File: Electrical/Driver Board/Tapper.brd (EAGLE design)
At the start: 71.9 x 31.4 mm, 30 parts, among them CN1 1X4-BIG, U10 DRV2605LDGS, U11 DRV2605LDGS, U12 TCA9548APWR, U3 DRV2605LDGS, U4 DRV2605LDGS, U5 DRV2605LDGS, U6 DRV2605LDGS, U7 DRV2605LDGS, U8 DRV2605LDGS, U9 DRV2605LDGS

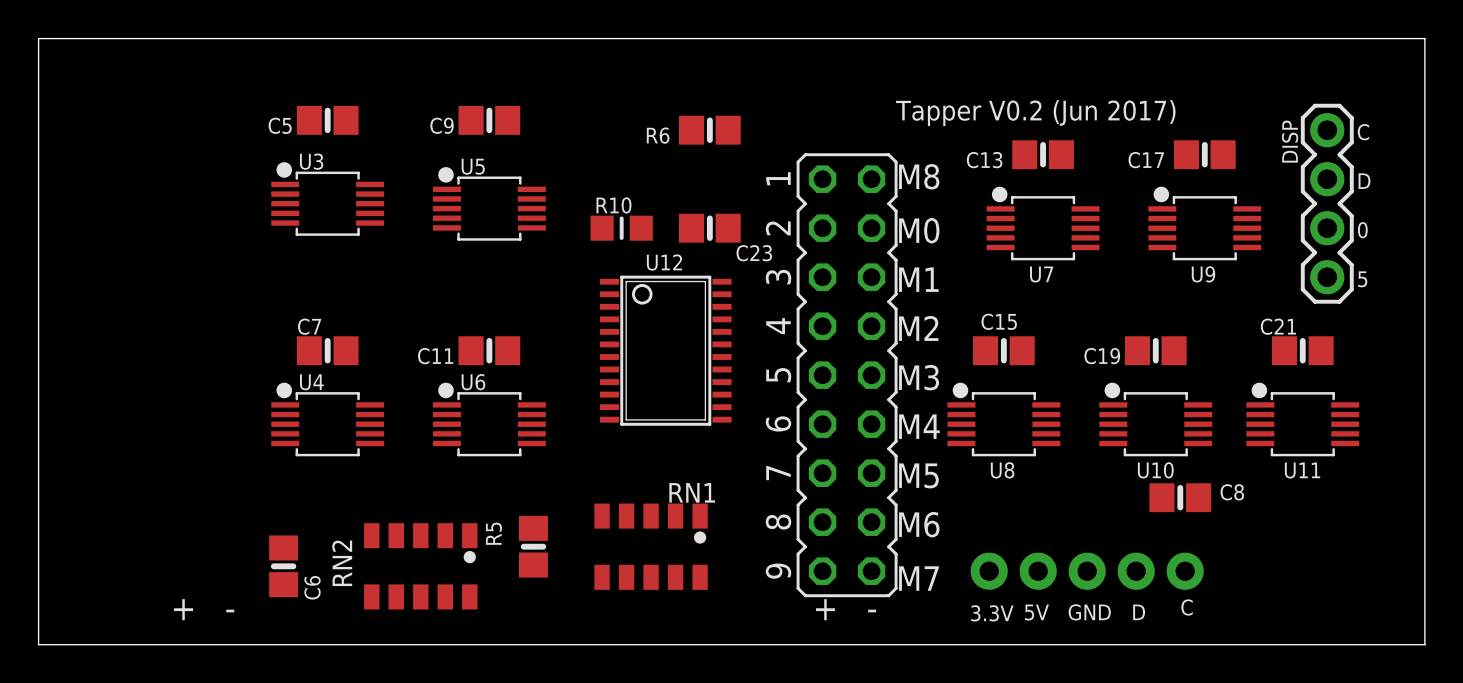
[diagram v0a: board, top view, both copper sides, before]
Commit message: .
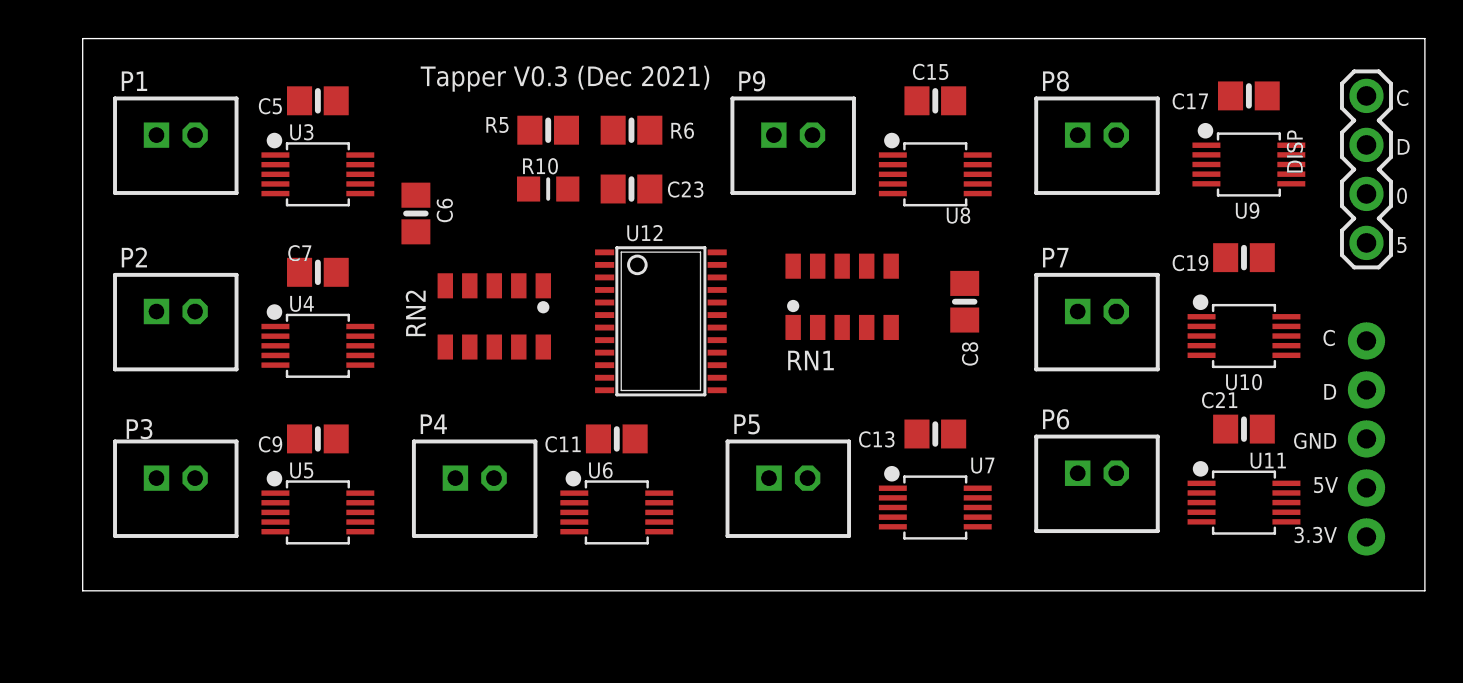
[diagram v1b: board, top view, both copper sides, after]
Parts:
- removed JP1: (no value), jumper:JP9Q
- added P1, P2, P3, P4, P5, P6, P7, P8, P9: B2B-PH-K, con-jst-ph:B2B-PH-K
- moved R5 21.6 mm to (15.0, 26.7), turned to 180 degrees
- moved C6 19.5 mm to (8.13, 22.4)
- moved C9 18.8 mm to (3.05, 10.7)
- moved U5 18.1 mm to (3.05, 6.86)
- moved RN1 16.3 mm to (30.2, 18.0), turned to 0 degrees
- moved JP2 16.0 mm to (57.4, 10.7), turned to 90 degrees
- moved U7 15.5 mm to (35.1, 7.11)
- moved C13 15.5 mm to (35.1, 10.9)
- moved C8 15.1 mm to (36.6, 17.8), turned to 270 degrees
- moved RN2 13.5 mm to (12.2, 17.0)
- moved U8 13.4 mm to (35.1, 24.4)
- moved C15 13.4 mm to (35.1, 28.2)
- moved C11 8.03 mm to (18.5, 10.7)
- moved U6 8.03 mm to (18.5, 6.86)
- moved C19 6.65 mm to (51.1, 20.1)
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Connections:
- net N$1: now also P2.2; no longer JP1.4
- net OUT+10: now also P6.1; no longer JP1.17
- net OUT+2: now also P1.1; no longer JP1.1
- net OUT+3: now also P2.1; no longer JP1.3
- net OUT+4: now also P3.1; no longer JP1.5
- net OUT+5: now also P4.1; no longer JP1.7
- net OUT+6: now also P5.1; no longer JP1.9
- net OUT+7: now also P9.1; no longer JP1.11
- net OUT+8: now also P8.1; no longer JP1.13
- net OUT+9: now also P7.1; no longer JP1.15
- net OUT-10: now also P6.2; no longer JP1.18
- net OUT-2: now also P1.2; no longer JP1.2
- net OUT-4: now also P3.2; no longer JP1.6
- net OUT-5: now also P4.2; no longer JP1.8
- net OUT-6: now also P5.2; no longer JP1.10
- net OUT-7: now also P9.2; no longer JP1.12
- net OUT-8: now also P8.2; no longer JP1.14
- net OUT-9: now also P7.2; no longer JP1.16
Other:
- board size 71.9 x 31.4 mm -> 69.6 x 28.6 mm
- board text added: "Tapper V0.3 (Dec 2021)"
- board text removed: "+"
- board text removed: "-"
- board text removed: "M0"
- board text removed: "M1"
- board text removed: "M2"
- board text removed: "M3"
- board text removed: "M4"
- board text removed: "M5"
- board text removed: "M6"
- board text removed: "M7"
- board text removed: "M8"
- board text removed: "Tapper V0.2 (Jun 2017)"
